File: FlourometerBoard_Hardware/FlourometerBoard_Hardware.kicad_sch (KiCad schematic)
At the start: 14 parts, among them J1 RJ45_LED_Shielded, J2 Conn_01x12_Pin, U1 Teensy4.1_DEV-16771, U2 OKI

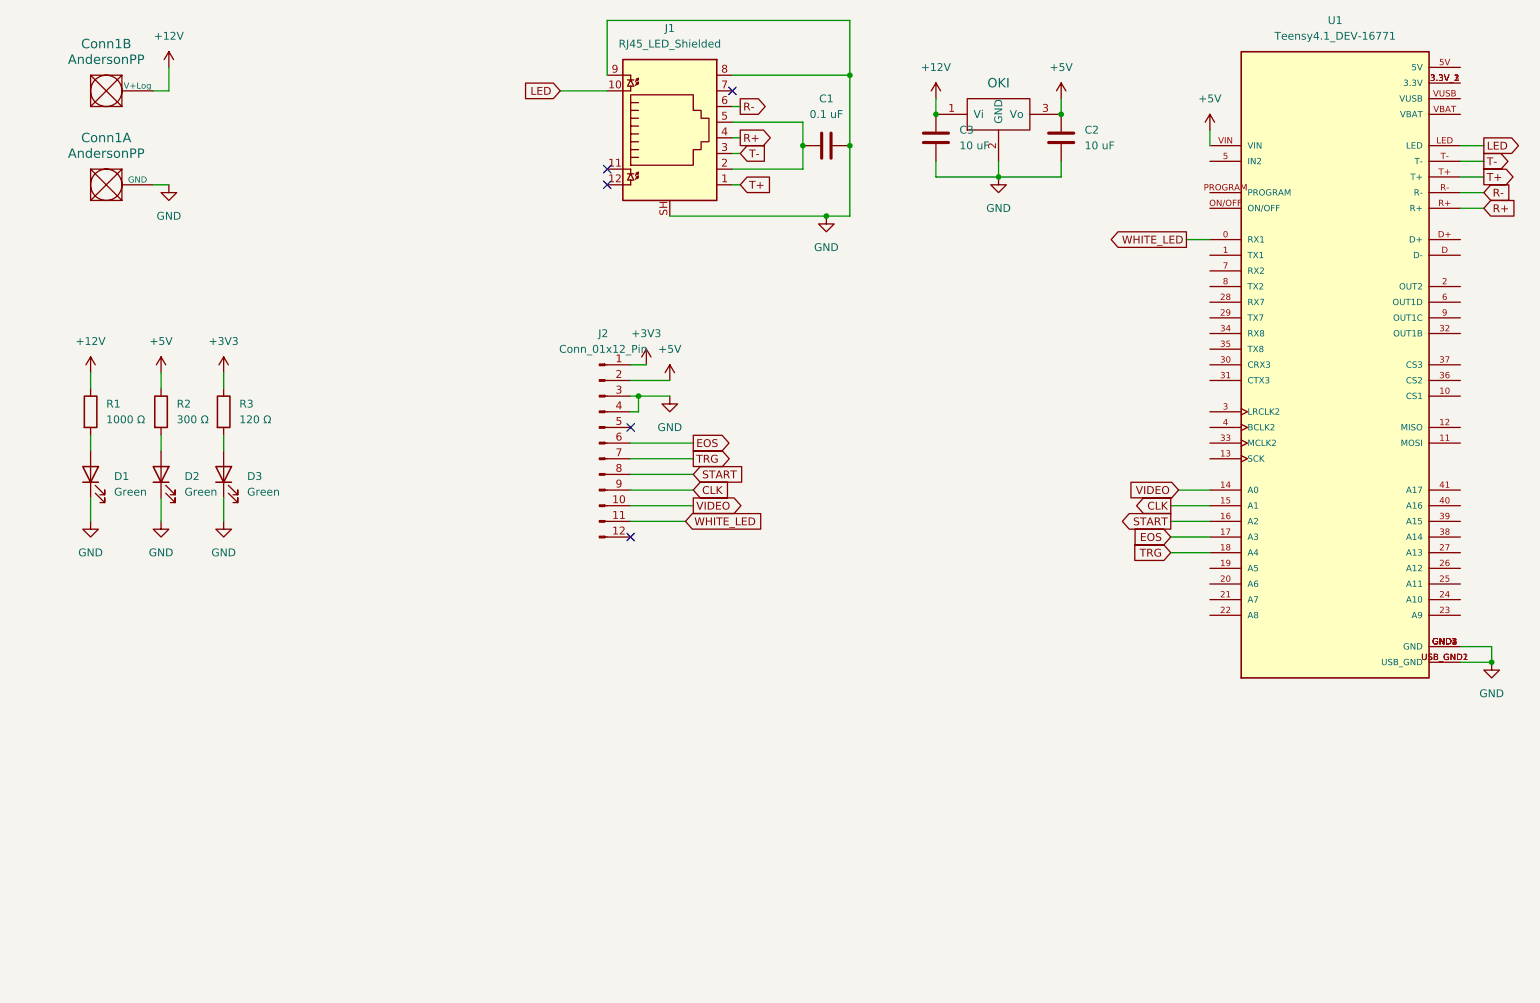
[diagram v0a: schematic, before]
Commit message: Boxed and Labeled Circuits
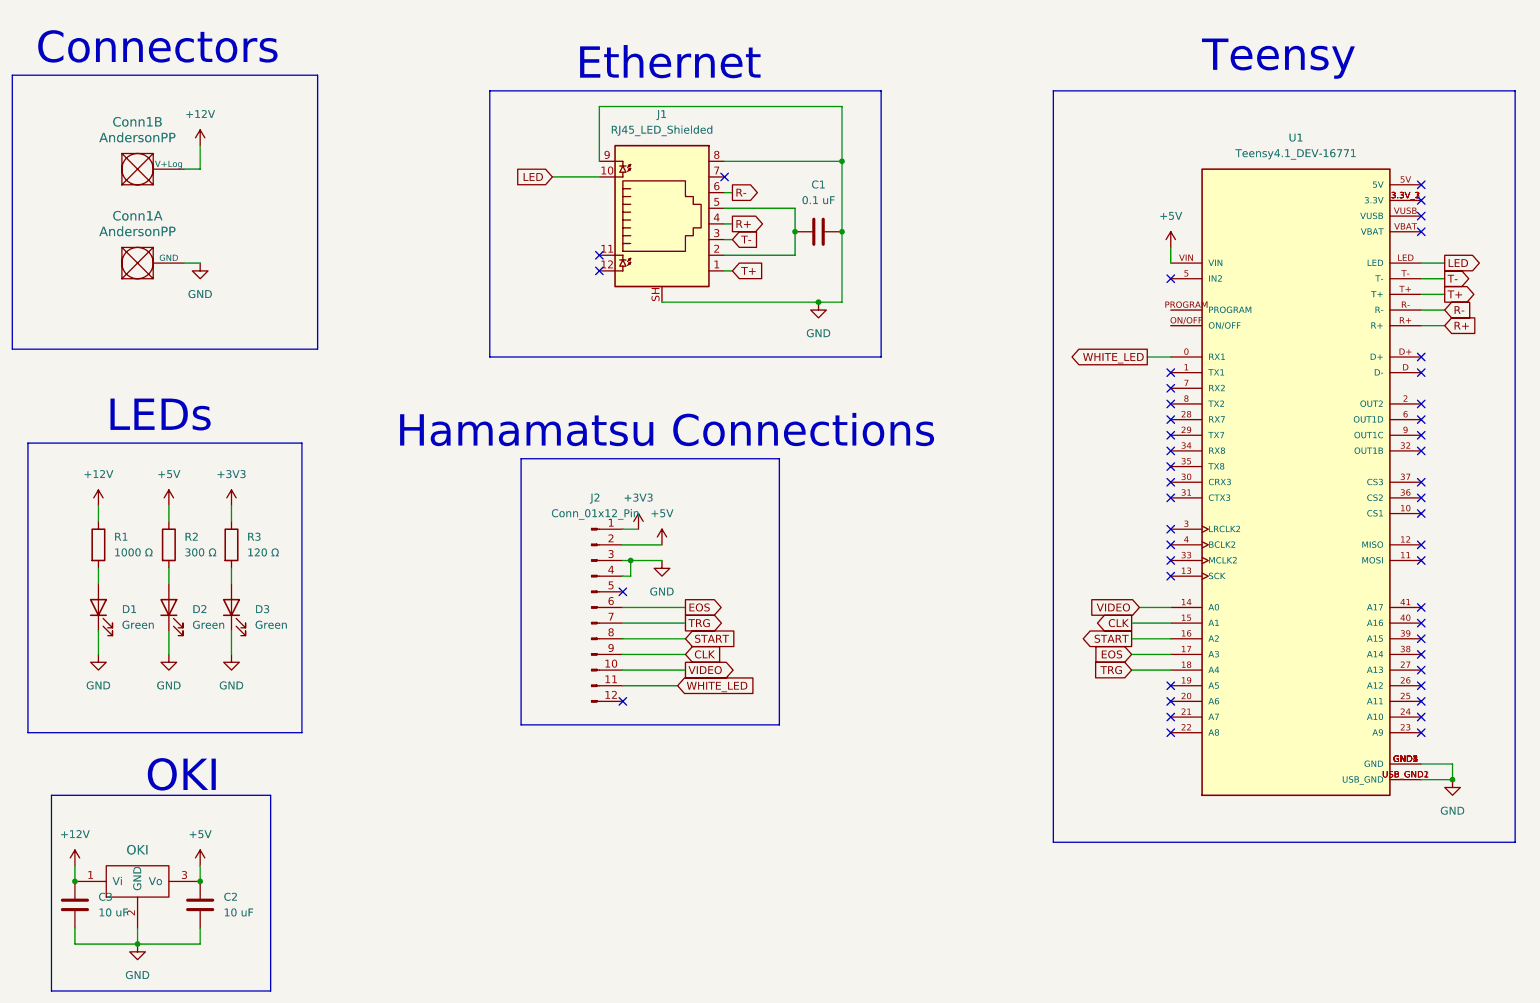
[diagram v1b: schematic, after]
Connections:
- no-connect marks 5 -> 47
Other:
- note added: "Connectors"
- note added: "Ethernet"
- note added: "Hamamatsu Connections"
- note added: "LEDs"
- note added: "OKI"
- note added: "Teensy"
- moved on the sheet: C1, C2, C3, Conn1A, Conn1B, D1, D2, D3, J1, J2, R1, R2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
